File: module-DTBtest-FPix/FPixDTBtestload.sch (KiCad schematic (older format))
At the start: 13 parts, among them J1 CONN-SMK20, P15 RTD+, P16 RTD-

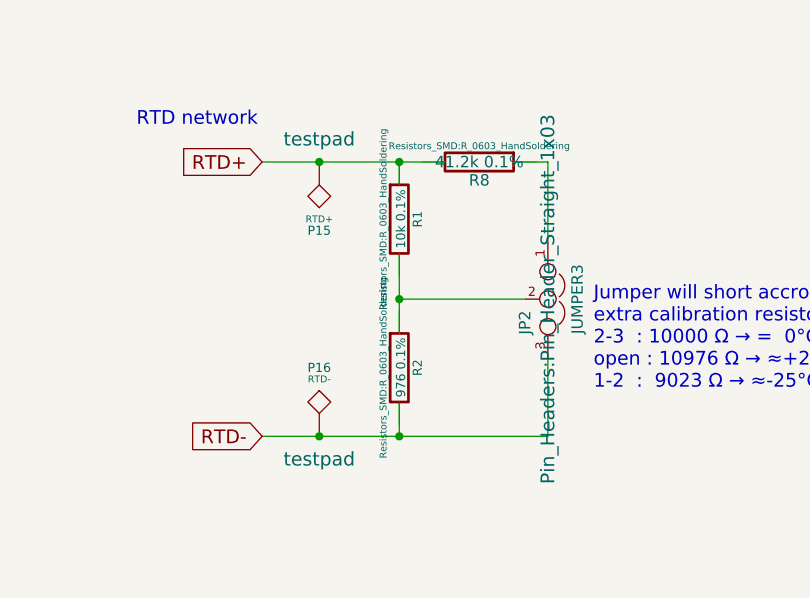
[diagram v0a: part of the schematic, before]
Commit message: first draft of potentially finished load board? please check
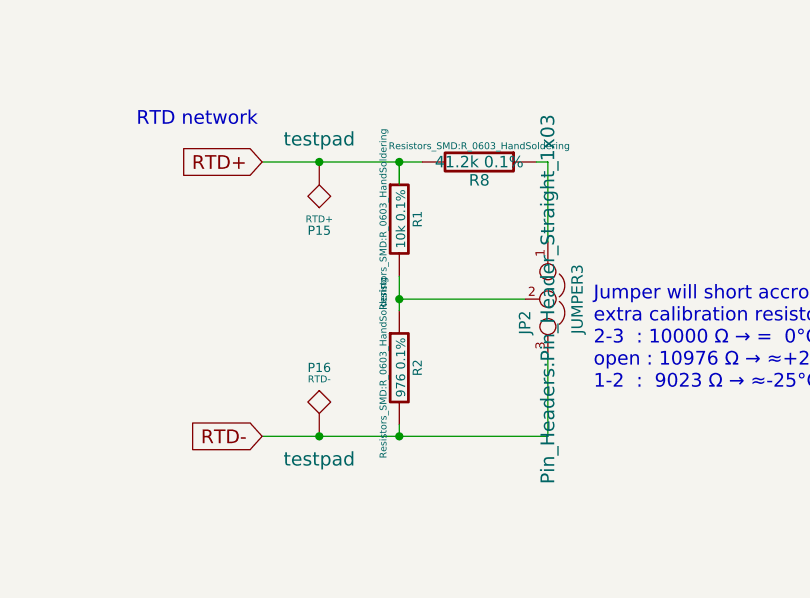
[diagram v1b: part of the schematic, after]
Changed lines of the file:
@@
 VD
 $Comp
-L GND #PWR?
+L GND #PWR09
 U 1 1 559D8FFC
 P 8700 4700
-F 0 "#PWR?" H 8700 4450 60  0001 C CNN
+F 0 "#PWR09" H 8700 4450 60  0001 C CNN
 F 1 "GND" H 8700 4550 60  0000 C CNN
 F 2 "" H 8700 4700 60  0000 C CNN
@@
 Text GLabel 7600 4650 0    60   Input ~ 0
 HV
-Connection ~ 7750 2300
 Connection ~ 7400 1100
 Connection ~ 7400 2300
@@
 	6550 5350 6400 5350
 Connection ~ 6550 5300
-Wire Wire Line
-	7150 1100 7950 1100
 Connection ~ 7750 1700
 Connection ~ 5650 5800
@@
 Wire Wire Line
 	7750 1100 7750 1200
-Wire Wire Line
-	7750 1500 7750 1850
-Wire Wire Line
-	7750 2300 7750 2150
 Wire Wire Line
 	7700 3500 7700 3400
@@
 Wire Wire Line
 	7750 1700 8300 1700
-Wire Wire Line
-	7150 2300 8400 2300
-Wire Wire Line
-	8400 2300 8400 1950
 Connection ~ 7750 1100
-Wire Wire Line
-	8250 1100 8400 1100
 Wire Wire Line
 	8400 1100 8400 1450
@@
 Wire Wire Line
 	7850 4650 7600 4650
+Wire Wire Line
+	7150 2300 8400 2300
+Wire Wire Line
+	7750 2300 7750 2250
+Wire Wire Line
+	8400 2300 8400 1950
+Connection ~ 7750 2300
+Wire Wire Line
+	7750 1600 7750 1750
+Wire Wire Line
+	7150 1100 7850 1100
+Wire Wire Line
+	8350 1100 8400 1100
 $EndSCHEMATC
